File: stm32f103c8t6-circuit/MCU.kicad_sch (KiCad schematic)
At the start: 13 parts, among them J7 Conn_01x04, SW1 , U1 STM32F103C8Tx, Y1 12M

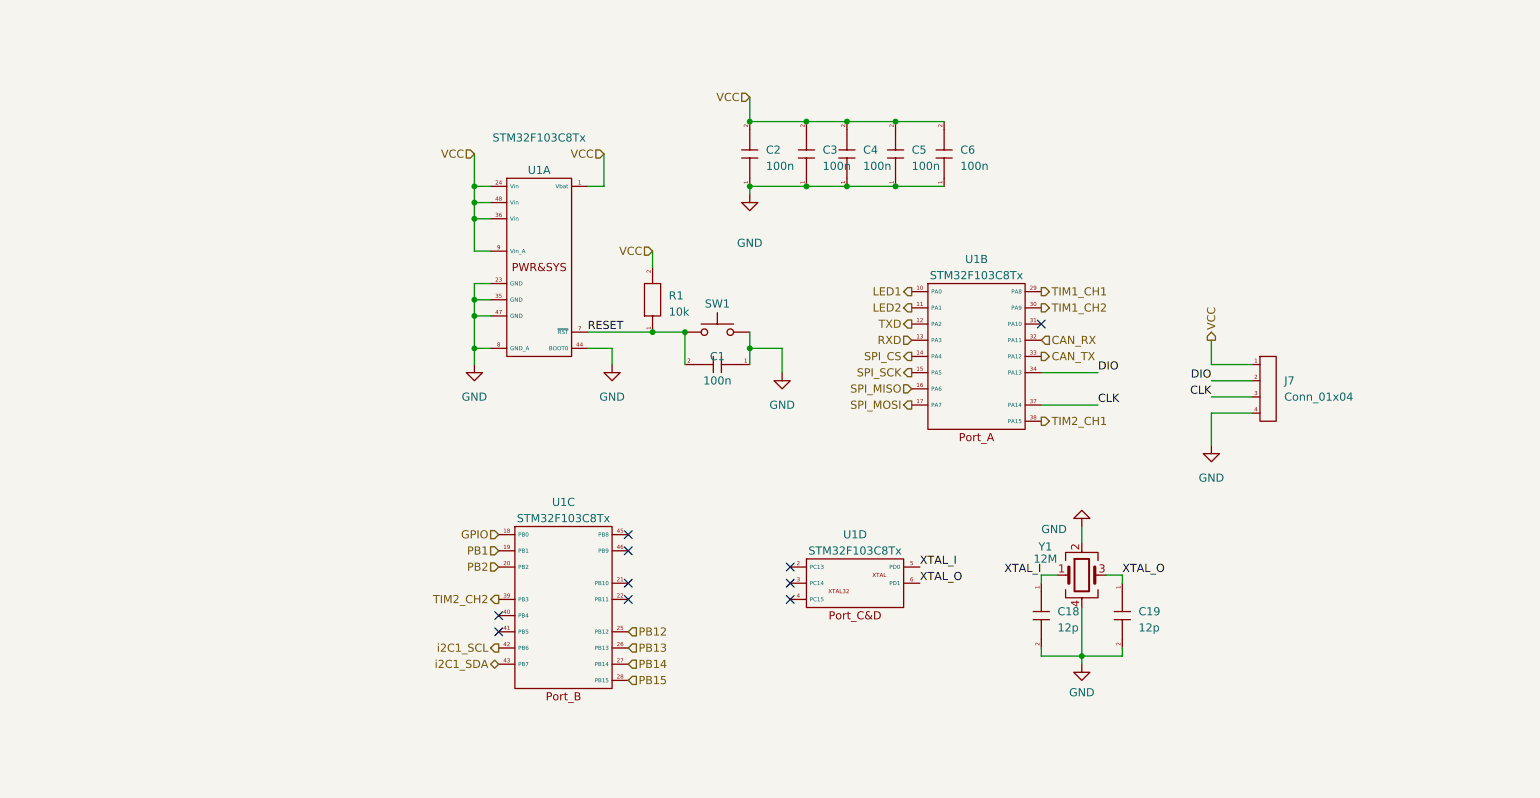
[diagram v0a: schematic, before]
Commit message: Modify PCH and SCH
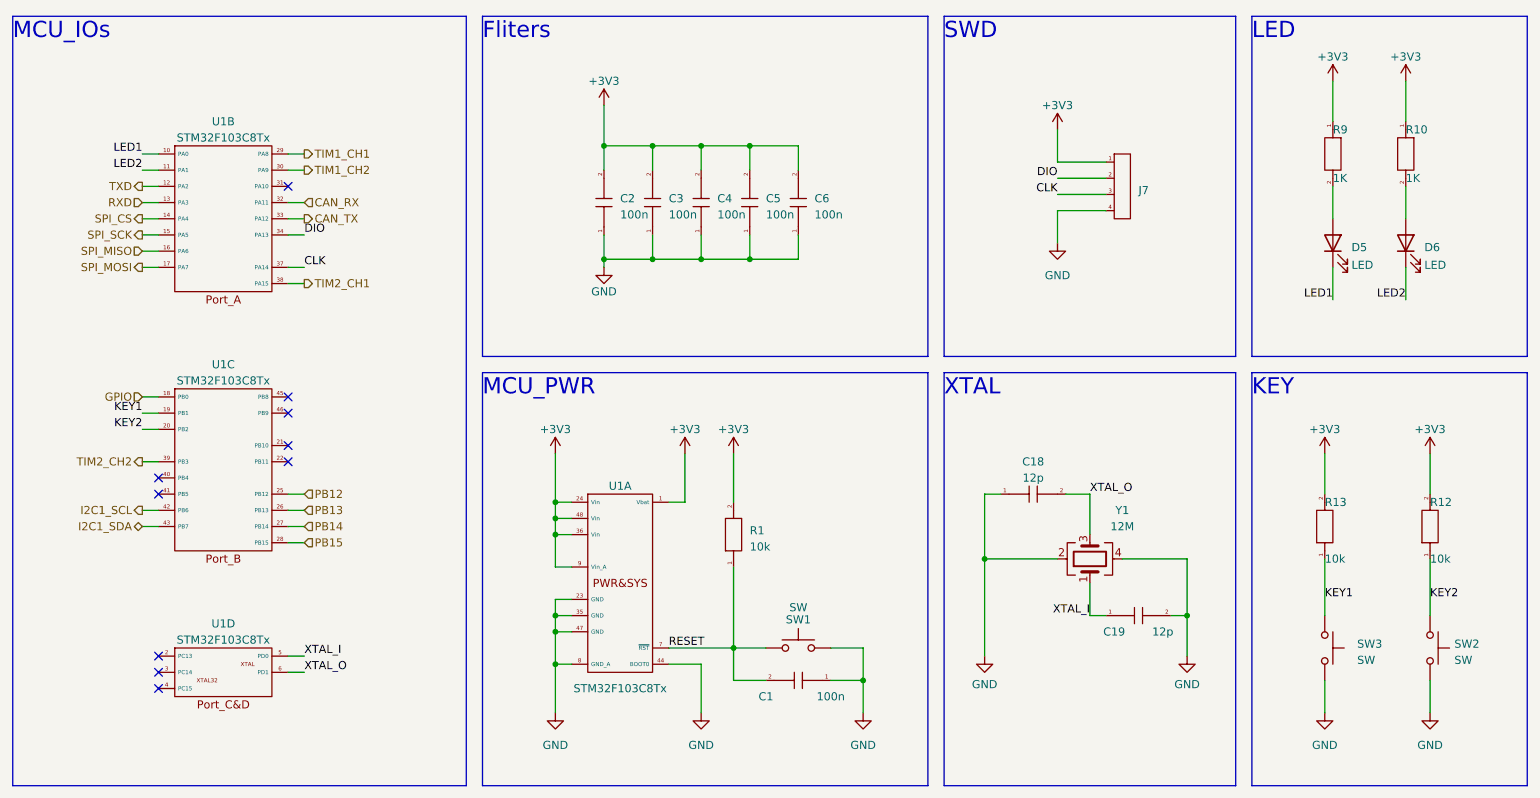
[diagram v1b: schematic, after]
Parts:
- added D5, D6: LED, LED_SMD:LED_0603_1608Metric, symbol Device:LED
- added R10, R9: 1K, ResistorSMD:R_0603_1608Metric, symbol 001_Basic_PassiveComponents:001_Resistor
- added R12, R13: 10k, ResistorSMD:R_0603_1608Metric, symbol 001_Basic_PassiveComponents:001_Resistor
- added SW2, SW3: SW, Button_Switch_SMD:SW_SPST_FSMSM, symbol Switch:SW_Push
- C1, C2, C3, C4, C5, C6: footprint PCM_001_GN_RCL_SMD:C0603(1608M) -> Capacitor_SMD:C_0603_1608Metric
- C18, C19: footprint Capacitor_SMD:C_0603_1608Metric_Pad1.08x0.95mm_HandSolder -> Capacitor_SMD:C_0603_1608Metric
- J7: footprint PCM_205_CONN_GH_SMD:GH1.25_H_4 -> Connector_PinHeader_2.54mm:PinHeader_1x04_P2.54mm_Vertical
- R1: footprint PCM_001_GN_RCL_SMD:R0603(1608M) -> ResistorSMD:R_0603_1608Metric
- SW1: value (none) -> SW
- U1: footprint PCM_004_GN_MIDDLE-SEMI_SMD:QFP-48_7070 -> PackageQFP:LQFP-48_7x7mm_P0.5mm
- Y1: footprint PCM_006_GN_XTAL_OSC_SMD:SMD-4_3225 -> Crystal:Crystal_SMD_3225-4Pin_3.2x2.5mm
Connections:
- net GND: now also C18.1, SW2.2, SW3.2; no longer C18.2
- net LED1: now also D5.1 (K)
- net LED2: now also D6.1 (K)
- net XTAL_I: now also C19.1; no longer C18.1
- net XTAL_O: now also C18.2; no longer C19.1
- net PB1 renamed KEY1
- net KEY1: now also R13.1, SW3.1
- net PB2 renamed KEY2
- net KEY2: now also R12.1, SW2.1
- net VCC renamed +3V3
- net +3V3: now also R10.1, R12.2, R13.2, R9.1
- net i2C1_SCL renamed I2C1_SCL
- net i2C1_SDA renamed I2C1_SDA
- new net: D6.2 (A), R10.2
- new net: D5.2 (A), R9.2
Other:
- note added: "Fliters"
- note added: "KEY"
- note added: "LED"
- note added: "MCU_IOs"
- note added: "MCU_PWR"
- note added: "SWD"
- note added: "XTAL"
- moved on the sheet: C1, C18, C19, C2, C3, C4, C5, C6, J7, R1, SW1, U1A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
